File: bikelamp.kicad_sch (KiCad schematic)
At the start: 18 parts, among them J1 Conn_ARM_SWD_TagConnect_TC203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, Q1 Q_PMOS_GSD, Q2 BSS138, SW1 SW_MEC_5E, U3 MIC5205-3.3YM5, U4 MMA8452QR1, U5 YJ-14015

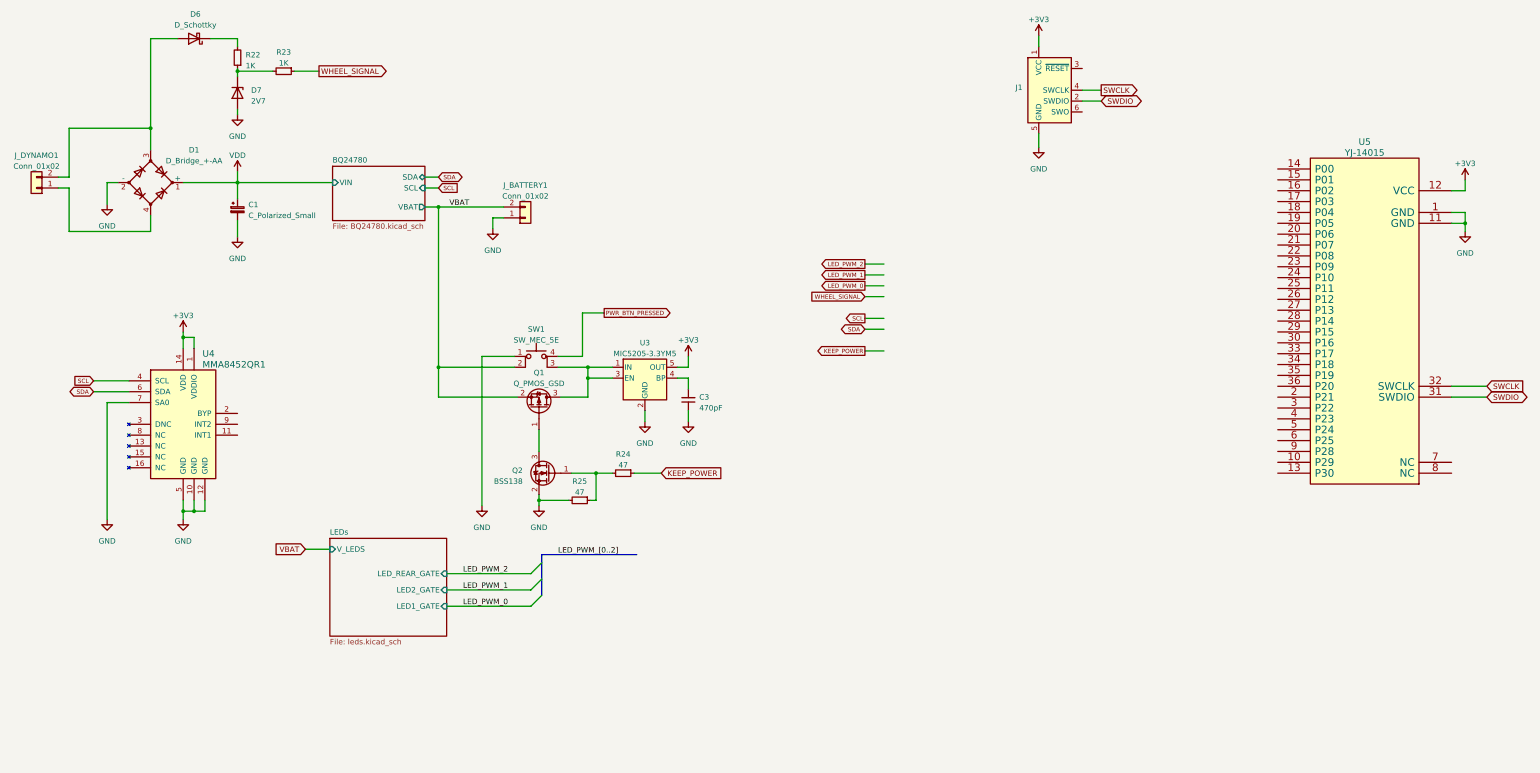
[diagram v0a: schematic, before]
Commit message: Working on contours
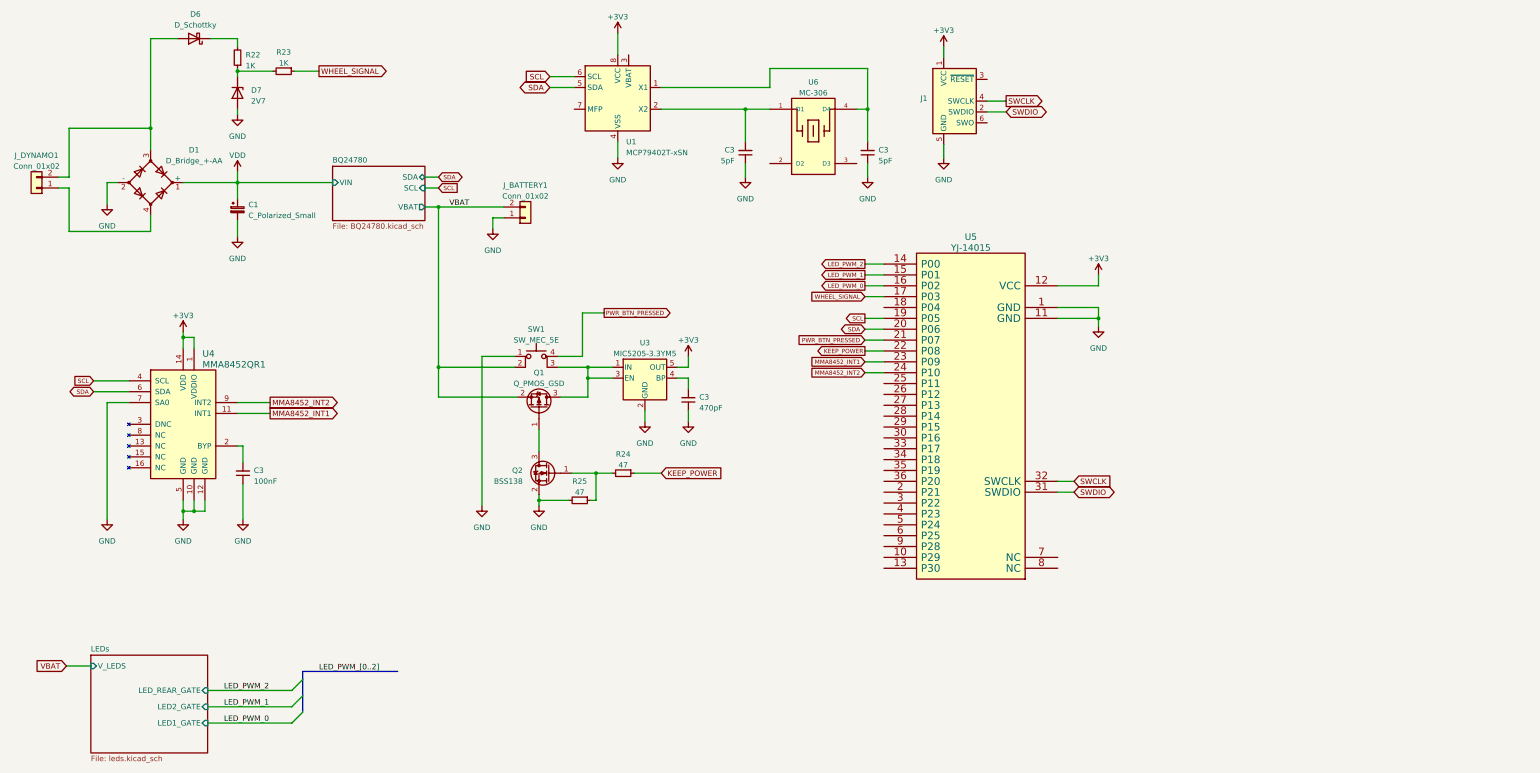
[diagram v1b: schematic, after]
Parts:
- added C3: 100nF, Capacitor_SMD:C_0603_1608Metric, symbol Device:C_Small
- added C3 (x2): 5pF, Capacitor_SMD:C_0603_1608Metric, symbol Device:C_Small
- added U1: MCP79402T-xSN, Package_SO:SO-8_3.9x4.9mm_P1.27mm, symbol Timer_RTC:MCP79402T-xSN
- added U6: MC-306, footprints:MC-306, symbol MC-306:MC-306
- C1: footprint (none) -> footprints:BQ24780SRUYR
- C3: footprint Resistor_SMD:R_0603_1608Metric -> Capacitor_SMD:C_0603_1608Metric
- R22, R23, R24, R25: footprint (none) -> Resistor_SMD:R_0603_1608Metric
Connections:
- net +3V3: now also U1.8 (VCC)
- net GND: now also C3.1, C3.1, C3.1, U1.4 (VSS)
- net KEEP_POWER: now also U5.22 (P08)
- net LED_PWM_0: now also U5.16 (P02)
- net LED_PWM_1: now also U5.15 (P01)
- net LED_PWM_2: now also U5.14 (P00)
- net PWR_BTN_PRESSED: now also U5.21 (P07)
- net SCL: now also U5.19 (P05), U1.6 (SCL)
- net SDA: now also U5.20 (P06), U1.5 (SDA)
- net WHEEL_SIGNAL: now also U5.17 (P03)
- net MMA8452_INT1: now reaches U4.11 (INT1)
- net MMA8452_INT1: now also U5.23 (P09)
- net at U4.2 (BYP): now also C3.2
- net MMA8452_INT2: now reaches U4.9 (INT2)
- net MMA8452_INT2: now also U5.24 (P10)
- new net: C3.2, U1.2 (X2), U6.1 (D1)
- new net: C3.2, U1.1 (X1), U6.4 (D4)
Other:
- moved on the sheet: J1, U5
